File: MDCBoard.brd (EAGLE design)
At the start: 43.9 x 32.6 mm, 200 parts, among them J1 JUMPER-SOLDER, J10 MICROSD-SOCKET, J11 USB-C-RECEPTACLE-KOREANHRO, J2 JUMPER-SOLDER, J3 JUMPER-SOLDER, J4 JUMPER-SOLDER, J5 JST-SM02B-SRSS-TB, J6 JUMPER-SOLDER, J7 JUMPER-SOLDER, J8 JUMPER-SOLDER, Q1 PMOS-NEXPERIA-SOT1220, Q2 PMOS-NEXPERIA-SOT1220, Q3 PMOS-NEXPERIA-SOT1220, Q4 DIODESINC-DMG2305UX, Q5 DIODESINC-DMG2305UX, Q6 DIODESINC-DMG2305UX, Q7 DIODESINC-DMG2305UX, Q8 DIODESINC-DMG2305UX, U1 TI-TPS2116, U10 TI-TPS22919DCK, U11 TI-TPS22919DCK, U12 TI-TPS22919DCK, U13 TI-TPS22919DCK, U14 TI-MSP430FR2422IRHL, U16 TI-TXB0102, U17 PANASONIC-EKMB110711X, U18 LATTICE-ICE40HX4K-BG121, U19 WINBOND-W25Q40EW, U2 DIODESINC-AP7350, U20 NEXPERIA-74LVC1G98-OR-INV-INP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, U21 NEXPERIA-74LVC1G98-BUFFER, U22 ON-AR0330CS1C12SPKA0, U23 ALLIANCE-AS4C8M16MSA-6BIN, U24 STM-STM32F730, U25 DIODESINC-DT1446-04V-7, U26 NEXPERIA-74LVC1G98-INVERTER, U3 NEXPERIA-74LVC1G98-NOR, U4 MICROCHIP-MCP7383X, U5 NEXPERIA-74LVC1G98-INVERTER, U6 EATON-STN101, U7 TI-TPS62A01, U8 TI-TPS62A01, U9 TI-TPS62A01, X1 EPSON-FC-135, X2 SITIME-SIT8021, X3 SITIME-SIT8021

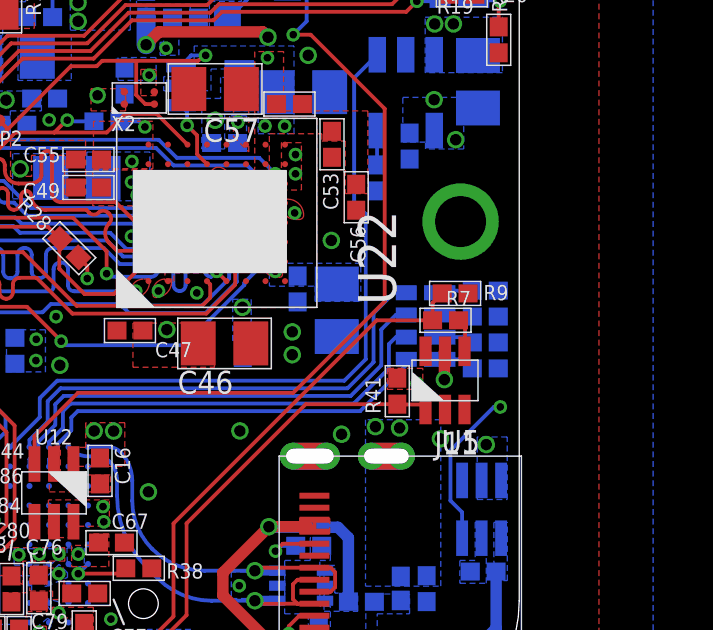
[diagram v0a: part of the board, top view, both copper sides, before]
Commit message: Layout progress
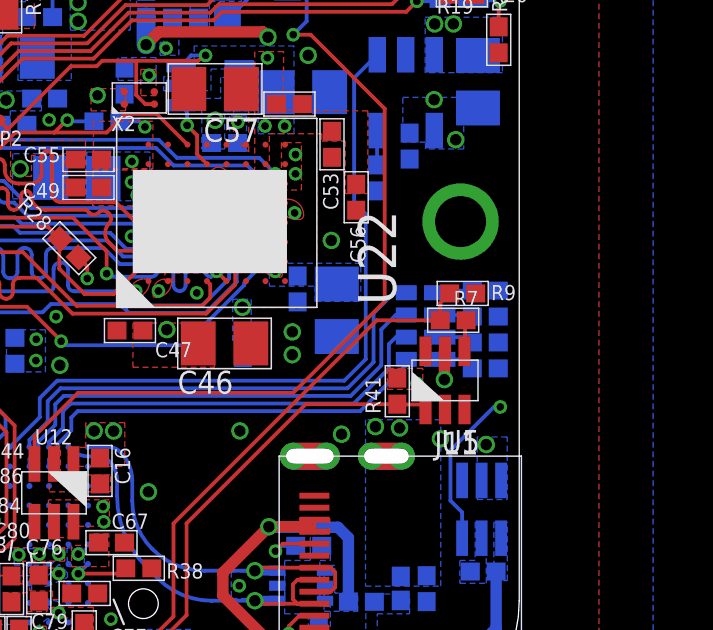
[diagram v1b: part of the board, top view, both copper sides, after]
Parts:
- moved R7 0.25 mm to (41.7, 14.1)
- moved R9 0.25 mm to (42.0, 15.0)
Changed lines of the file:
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@@
 <attribute name="PN" value="74LVC1G98GW,125" x="41.381021875" y="12.097940625" size="1.778" layer="27" rot="R90" display="off"/>
 </element>
-<element name="R9" library="EagleLibrary" package="0402" value="300k" x="41.717096875" y="14.997796875" smashed="yes">
-<attribute name="MFG" value="Walsin" x="41.717096875" y="14.997796875" size="1.778" layer="27" display="off"/>
-<attribute name="NAME" x="42.659815625" y="14.771475" size="0.508" layer="25" font="vector"/>
-<attribute name="PN" value="WR04X3003FTL" x="41.717096875" y="14.997796875" size="1.778" layer="27" display="off"/>
+<element name="R9" library="EagleLibrary" package="0402" value="300k" x="41.971096875" y="14.997796875" smashed="yes">
+<attribute name="MFG" value="Walsin" x="41.971096875" y="14.997796875" size="1.778" layer="27" display="off"/>
+<attribute name="NAME" x="42.913815625" y="14.771475" size="0.508" layer="25" font="vector"/>
+<attribute name="PN" value="WR04X3003FTL" x="41.971096875" y="14.997796875" size="1.778" layer="27" display="off"/>
 </element>
-<element name="R7" library="EagleLibrary" package="0402" value="100k" x="41.398884375" y="14.100478125" smashed="yes" rot="R180">
-<attribute name="MFG" value="Yageo" x="41.398884375" y="14.100478125" size="1.778" layer="27" rot="R180" display="off"/>
-<attribute name="NAME" x="42.246865625" y="15.08625625" size="0.508" layer="25" font="vector" rot="R180"/>
-<attribute name="PN" value="RC0402FR-07100KL" x="41.398884375" y="14.100478125" size="1.778" layer="27" rot="R180" display="off"/>
+<element name="R7" library="EagleLibrary" package="0402" value="100k" x="41.652884375" y="14.100478125" smashed="yes" rot="R180">
+<attribute name="MFG" value="Yageo" x="41.652884375" y="14.100478125" size="1.778" layer="27" rot="R180" display="off"/>
+<attribute name="NAME" x="42.500865625" y="15.08625625" size="0.508" layer="25" font="vector" rot="R180"/>
+<attribute name="PN" value="RC0402FR-07100KL" x="41.652884375" y="14.100478125" size="1.778" layer="27" rot="R180" display="off"/>
 </element>
 <element name="C7" library="EagleLibrary" package="0402" value="100n" x="20.17004375" y="4.555859375" smashed="yes" rot="R180">
@@
 <contactref element="R7" pad="2"/>
 <wire x1="32.330146875" y1="7.3286" x2="39.102025" y2="14.100478125" width="0.127" layer="1"/>
-<wire x1="39.102025" y1="14.100478125" x2="40.966384375" y2="14.100478125" width="0.127" layer="1"/>
+<wire x1="39.102025" y1="14.100478125" x2="41.220384375" y2="14.100478125" width="0.127" layer="1"/>
 <wire x1="32.330146875" y1="4.228225" x2="28.80653125" y2="0.704609375" width="0.127" layer="1"/>
 <wire x1="32.330146875" y1="4.228225" x2="32.330146875" y2="7.3286" width="0.127" layer="1"/>
@@
 <wire x1="18.191084375" y1="0.71881875" x2="18.533978125" y2="1.0617125" width="0.127" layer="1"/>
 <wire x1="14.02161875" y1="0.71881875" x2="18.191084375" y2="0.71881875" width="0.127" layer="1"/>
-<wire x1="41.284596875" y1="14.997796875" x2="40.966384375" y2="14.679584375" width="0.127" layer="1"/>
-<wire x1="40.966384375" y1="14.679584375" x2="40.966384375" y2="14.100478125" width="0.127" layer="1"/>
+<wire x1="41.538596875" y1="14.997796875" x2="41.220384375" y2="14.679584375" width="0.127" layer="1"/>
+<wire x1="41.220384375" y1="14.679584375" x2="41.220384375" y2="14.100478125" width="0.127" layer="1"/>
 <wire x1="23.933090625" y1="0.704609375" x2="20.60254375" y2="4.03515625" width="0.127" layer="1"/>
 <wire x1="20.60254375" y1="4.03515625" x2="20.60254375" y2="4.555859375" width="0.127" layer="1"/>
@@
 <contactref element="R7" pad="1"/>
 <wire x1="42.031021875" y1="13.068340625" x2="42.049821875" y2="13.087140625" width="0.127" layer="1"/>
-<wire x1="42.049821875" y1="13.087140625" x2="42.049821875" y2="13.882040625" width="0.127" layer="1"/>
-<wire x1="42.049821875" y1="13.882040625" x2="41.831384375" y2="14.100478125" width="0.127" layer="1"/>
+<wire x1="42.049821875" y1="13.087140625" x2="42.049821875" y2="14.064915625" width="0.127" layer="1"/>
+<wire x1="42.049821875" y1="14.064915625" x2="42.085384375" y2="14.100478125" width="0.127" layer="1"/>
 </signal>
 <signal name="MSP_HOST_MODE_">
